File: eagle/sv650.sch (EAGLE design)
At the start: 17 parts, among them IC1 7805

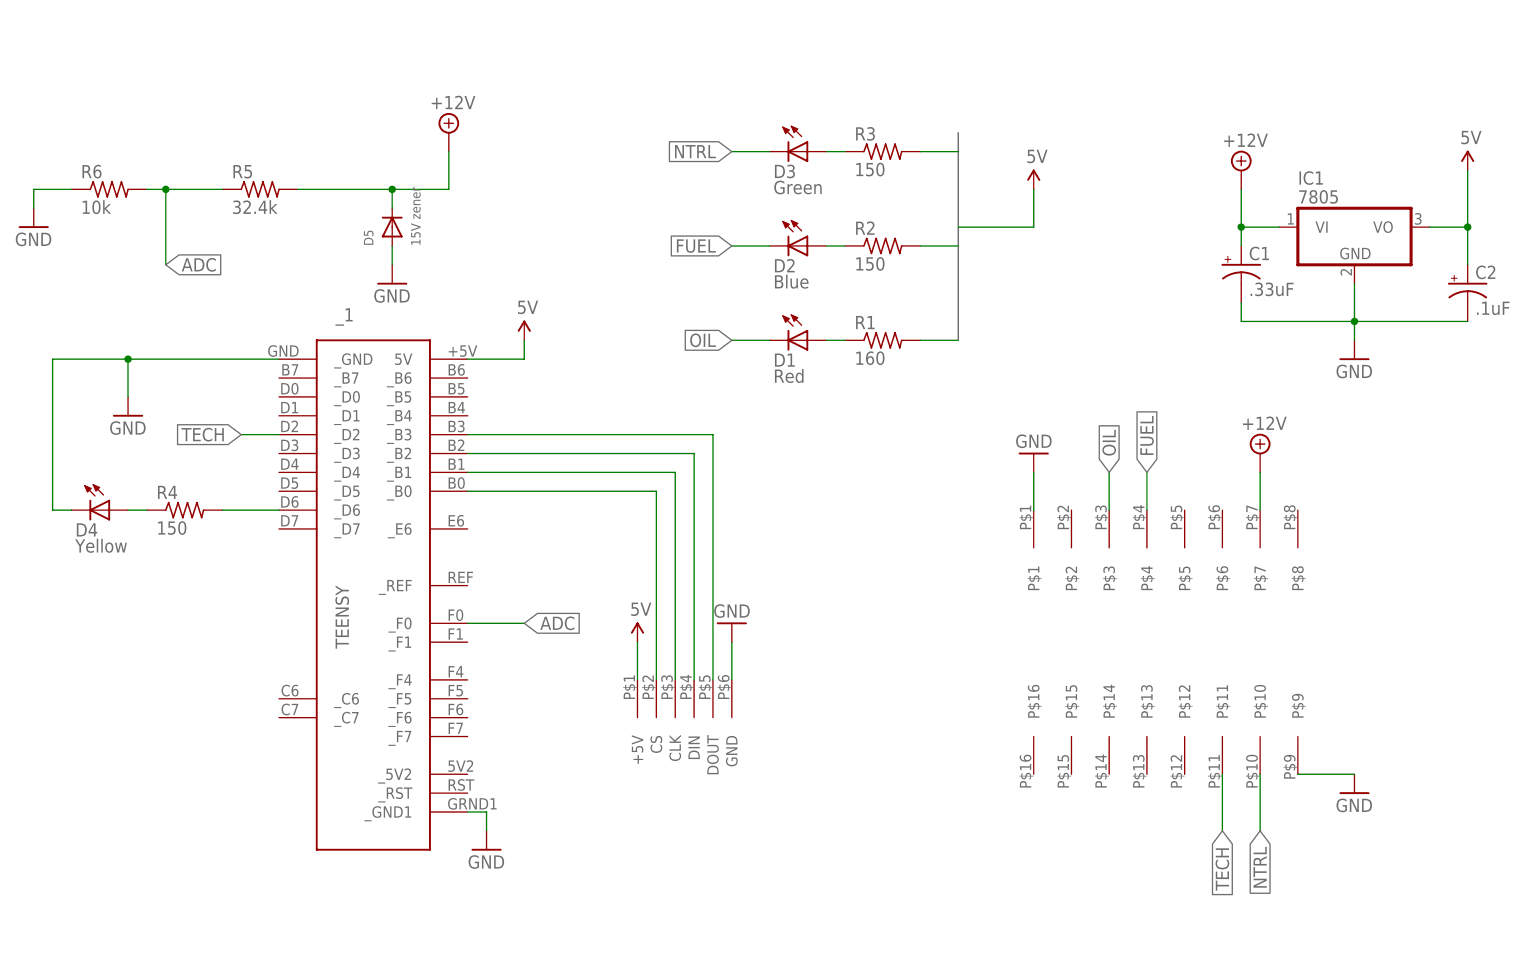
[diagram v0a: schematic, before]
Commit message: board as ordered from OshPark for v4.0
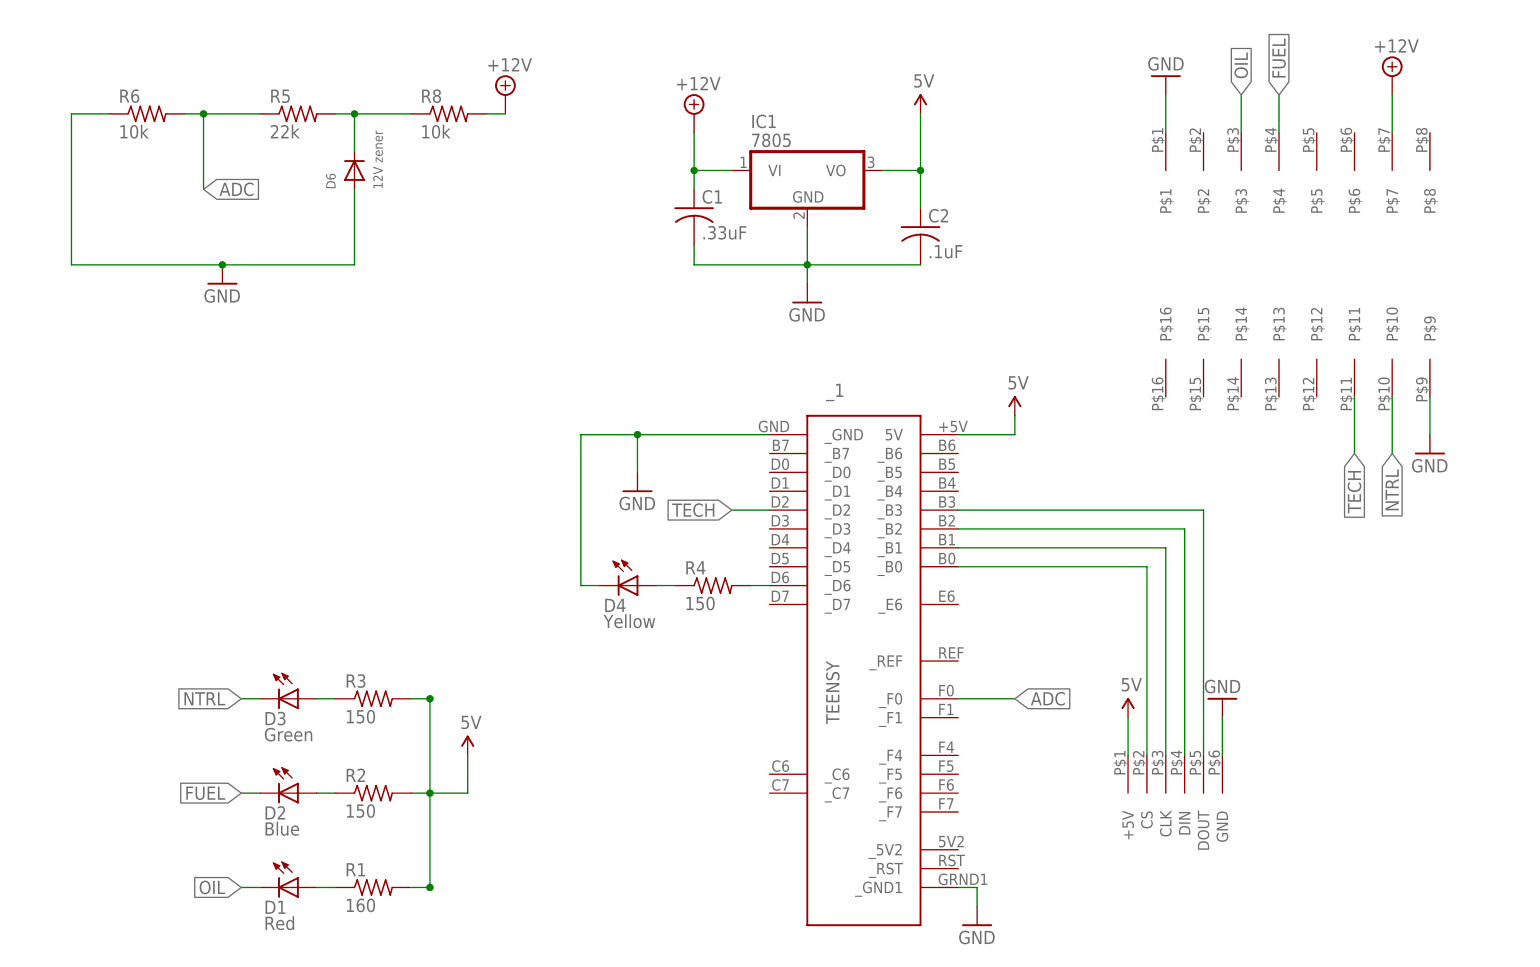
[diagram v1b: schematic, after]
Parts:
- removed D5: 15V zener, adafruit:DIODESOD-123
- added D6: 12V zener, adafruit:DIODESOD-123
- added R8: 10k, resistor:R-US_M0805
- C1, C2: device SparkFun:CAP_POL1206 -> adafruit:C-US025-024X044
- R1: MF (none) -> VISHAY/DALE; MPN (none) -> CRCW0805160RFKEA; OC_NEWARK unknown -> 52K9907
- R2, R3, R4: MPN (none) -> MCHP05W4F1500T5E; OC_NEWARK unknown -> 01N7000
- R5: value 32.4k -> 22k; MPN (none) -> CRCW080522K0FKEA; OC_NEWARK unknown -> 61M5466
- R6: MF (none) -> VISHAY/DALE; MPN (none) -> CRCW080510K0FKTA; OC_NEWARK unknown -> 05F1511
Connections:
- new net N$13: D6.C, R5.2, R8.1
- net +12V: now also C1.1, R8.2; no longer C1.+, D5.C, R5.2
- net 5V: now also C2.1; no longer C2.+
- net GND: now also C1.2, C2.2, D6.A; no longer C1.-, C2.-, D5.A
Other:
- moved on the sheet: D1, D2, D3, D4, IC1, R1, R2, R3, R4, R5, R6, _1
